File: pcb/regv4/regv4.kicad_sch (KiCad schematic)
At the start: 21 parts, among them J1 RST, J101 DATA_IN, J102 DATA_OUT, J103 WR_EN, J104 CLK, J105 +5V, J106 GND, Q101 MMBT3904, Q102 MMBT3904, Q103 MMBT3904, Q25 MMBT3904, Q26 MMBT3904

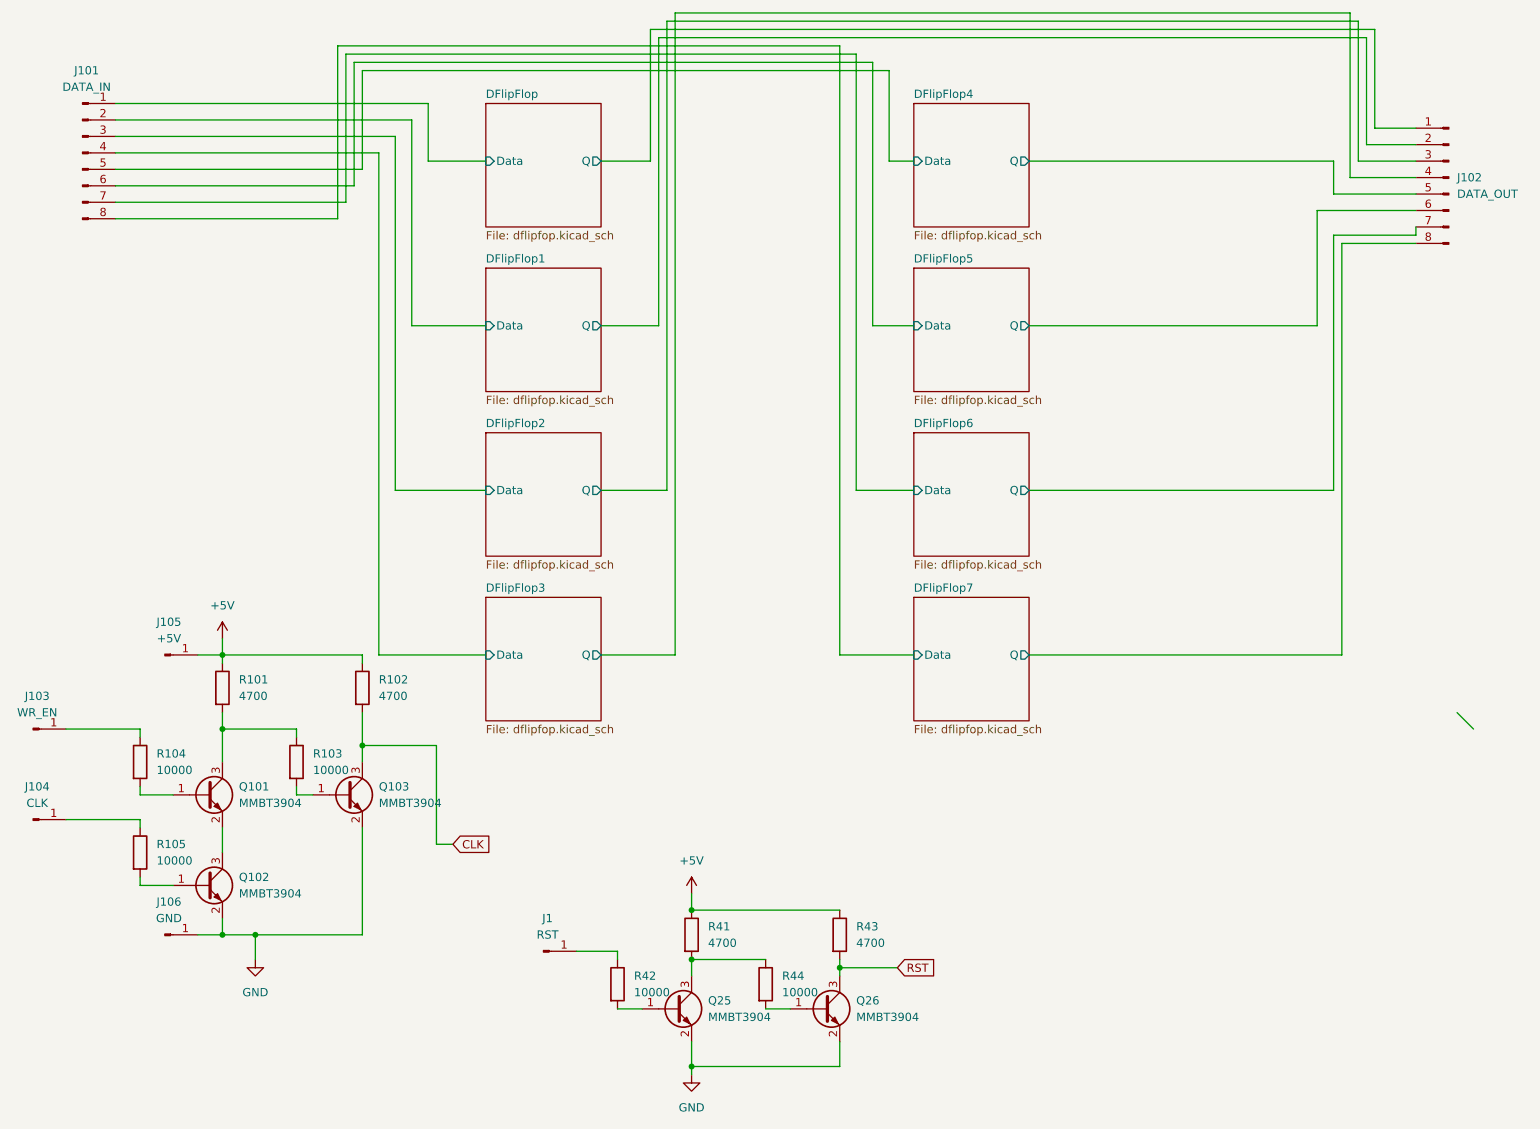
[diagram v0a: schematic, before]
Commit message: small work on regv4 (so lazy)
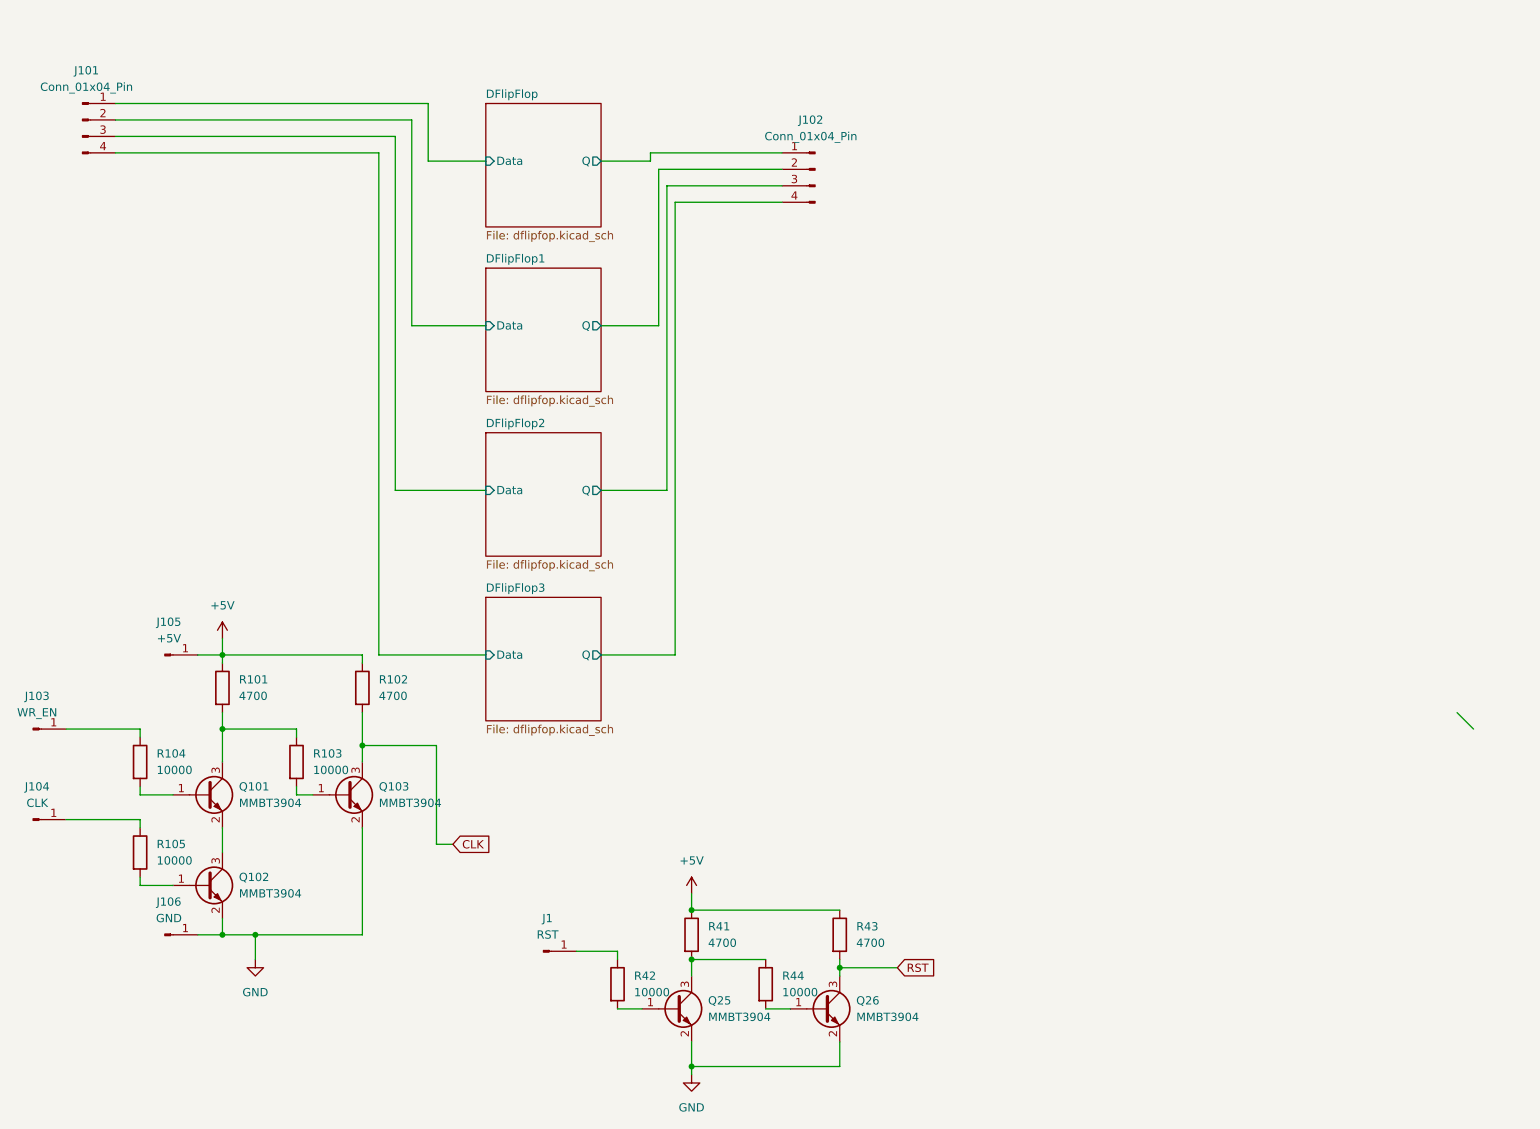
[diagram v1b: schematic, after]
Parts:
- removed J101: DATA_IN, Connector_PinHeader_2.54mm:PinHeader_1x08_P2.54mm_Vertical, symbol Connector:Conn_01x08_Pin
- removed J102: DATA_OUT, Connector_PinHeader_2.54mm:PinHeader_1x08_P2.54mm_Vertical, symbol Connector:Conn_01x08_Pin
- added J101, J102: Conn_01x04_Pin, Connector_PinHeader_2.54mm:PinHeader_1x04_P2.54mm_Vertical, symbol Connector:Conn_01x04_Pin
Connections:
- net DFlipFlop/Data: now also J101.1 (Pin_1)
- net DFlipFlop/Q: now also J102.1 (Pin_1)
- net DFlipFlop1/Data: now also J101.2 (Pin_2)
- net DFlipFlop1/Q: now also J102.2 (Pin_2)
- net DFlipFlop2/Data: now also J101.3 (Pin_3)
- net DFlipFlop2/Q: now also J102.3 (Pin_3)
- net DFlipFlop3/Data: now also J101.4 (Pin_4)
- net DFlipFlop3/Q: now also J102.4 (Pin_4)
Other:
- removed sheet DFlipFlop4
- removed sheet DFlipFlop5
- removed sheet DFlipFlop6
- removed sheet DFlipFlop7
